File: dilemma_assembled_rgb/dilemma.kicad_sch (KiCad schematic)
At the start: 92 parts, among them J1 USB_C_Receptacle_USB2.0, J102 Serial, J105 Conn_01x04_Female, J113 Cirque, J2 Conn_01x03_Female, J5 Conn_01x02, SW1 SW_Push, SW110 SW_SPST, SW2 SW_Push, SW3002 RotaryEncoder_Switch, U1 RP2040, U2 GD25Q80CEIGR, U3 XC6210B332MR-G, U4 USBLC6-2P6, Y1 Crystal_GND24

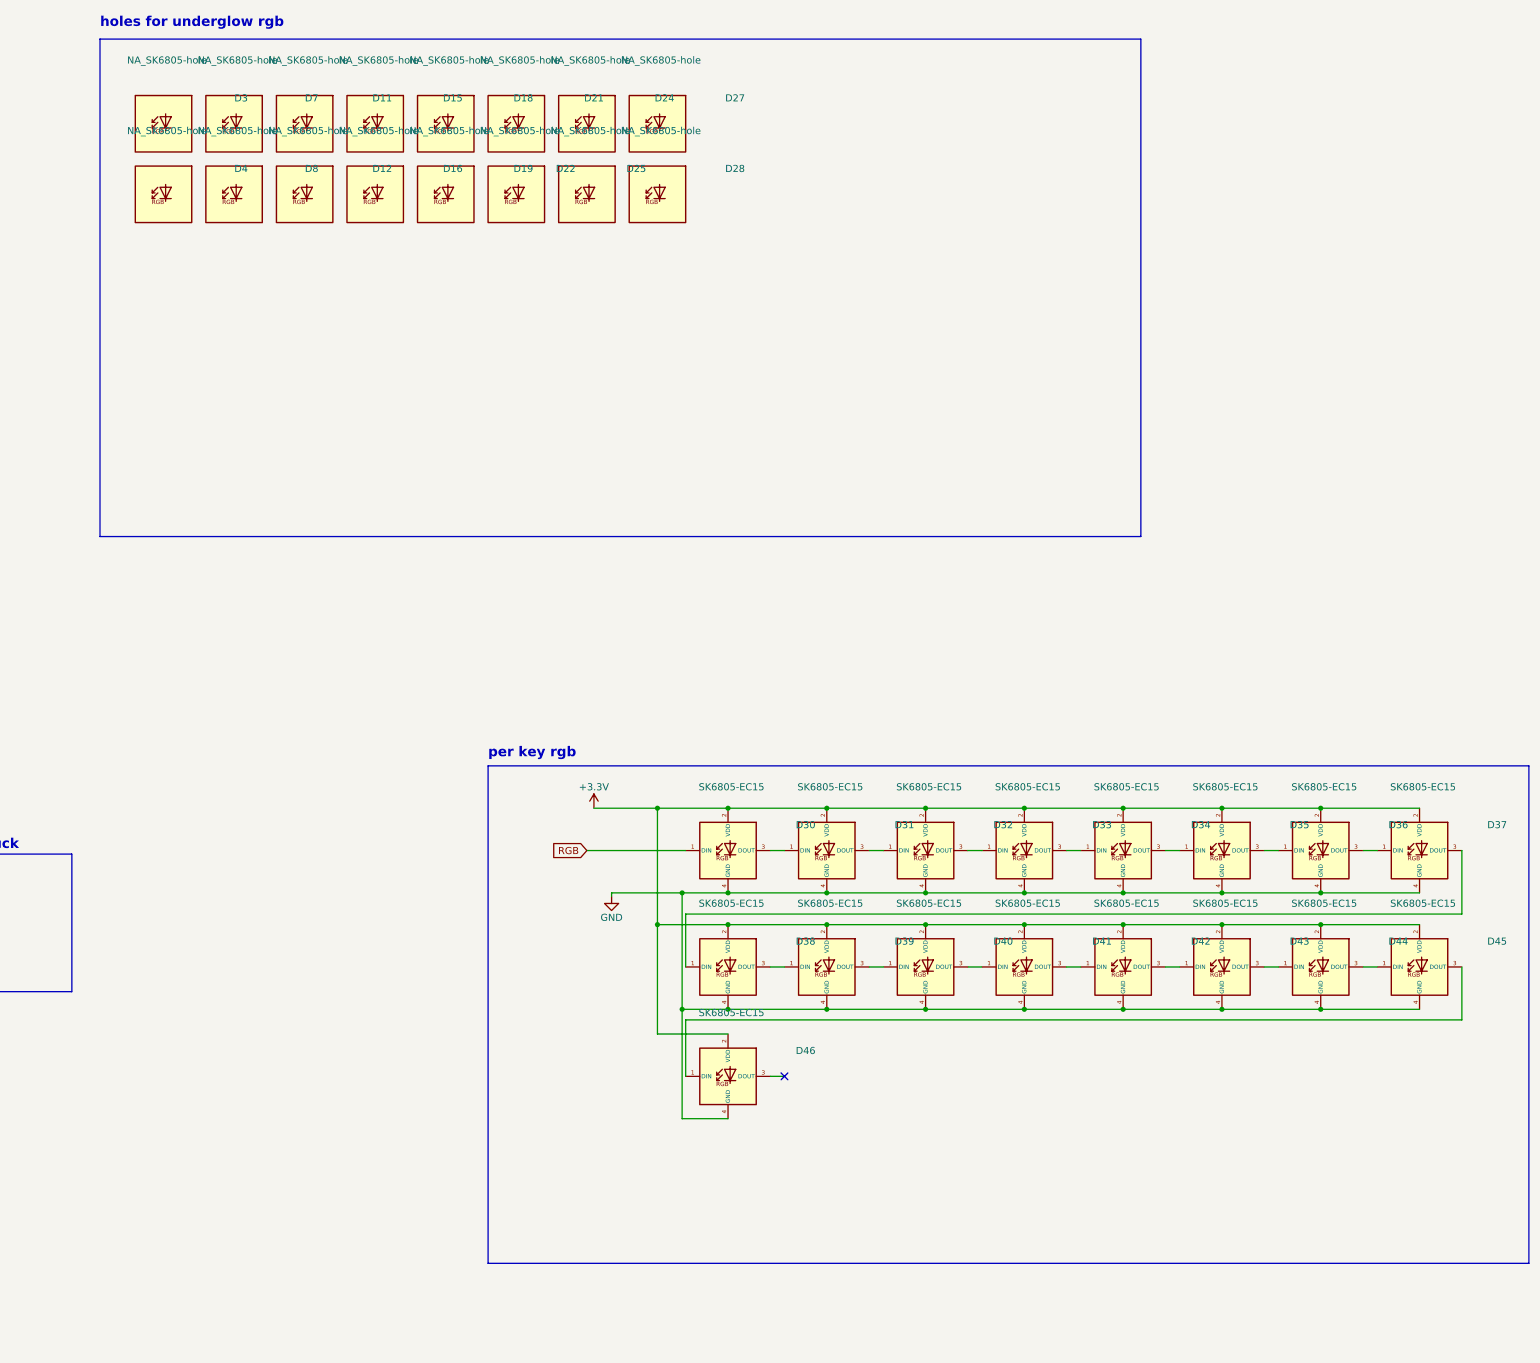
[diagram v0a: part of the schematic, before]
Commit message: cleanup
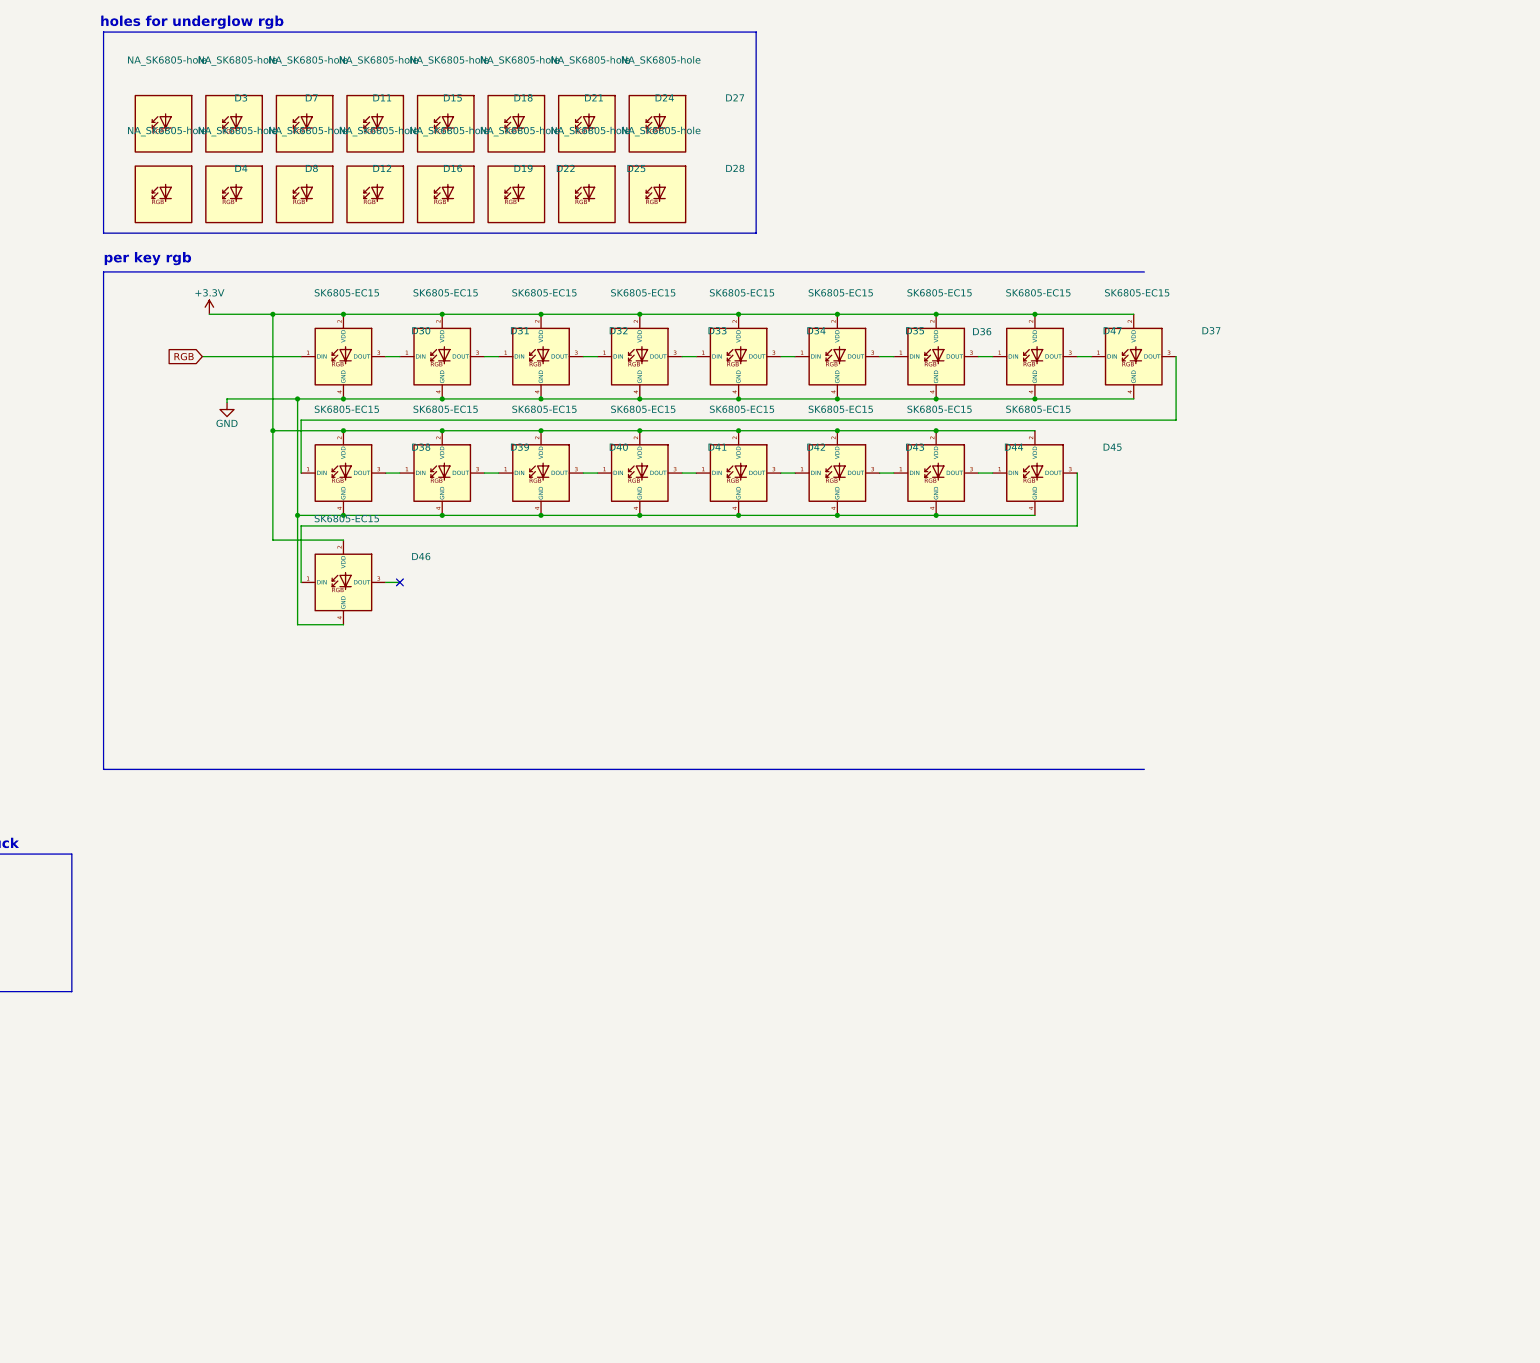
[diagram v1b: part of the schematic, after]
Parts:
- added D47: SK6805-EC15, local-libraries:LED_SK6805-EC15_withSwitch, symbol sk6805-ec15:SK6805-EC15
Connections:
- net +3V3: now also D47.2 (VDD)
- net GND: now also D47.4 (GND)
- net at D36.3 (DOUT): now also D47.1 (DIN); no longer D37.1 (DIN)
- new net: D37.1 (DIN), D47.3 (DOUT)
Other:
- moved on the sheet: D30, D31, D32, D33, D34, D35, D36, D37, D38, D39, D40, D41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
